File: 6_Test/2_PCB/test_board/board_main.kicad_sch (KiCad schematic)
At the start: 20 parts, among them J1 Power_Connector, J2 BNC_Odd, J3 BNC_Even, J4 Analog_Discovery_Inputs, J5 BNC_Inputs, J7 Digital_Supply_Jumpers, J8 Digital_Outputs, J9 Digital_Inputs

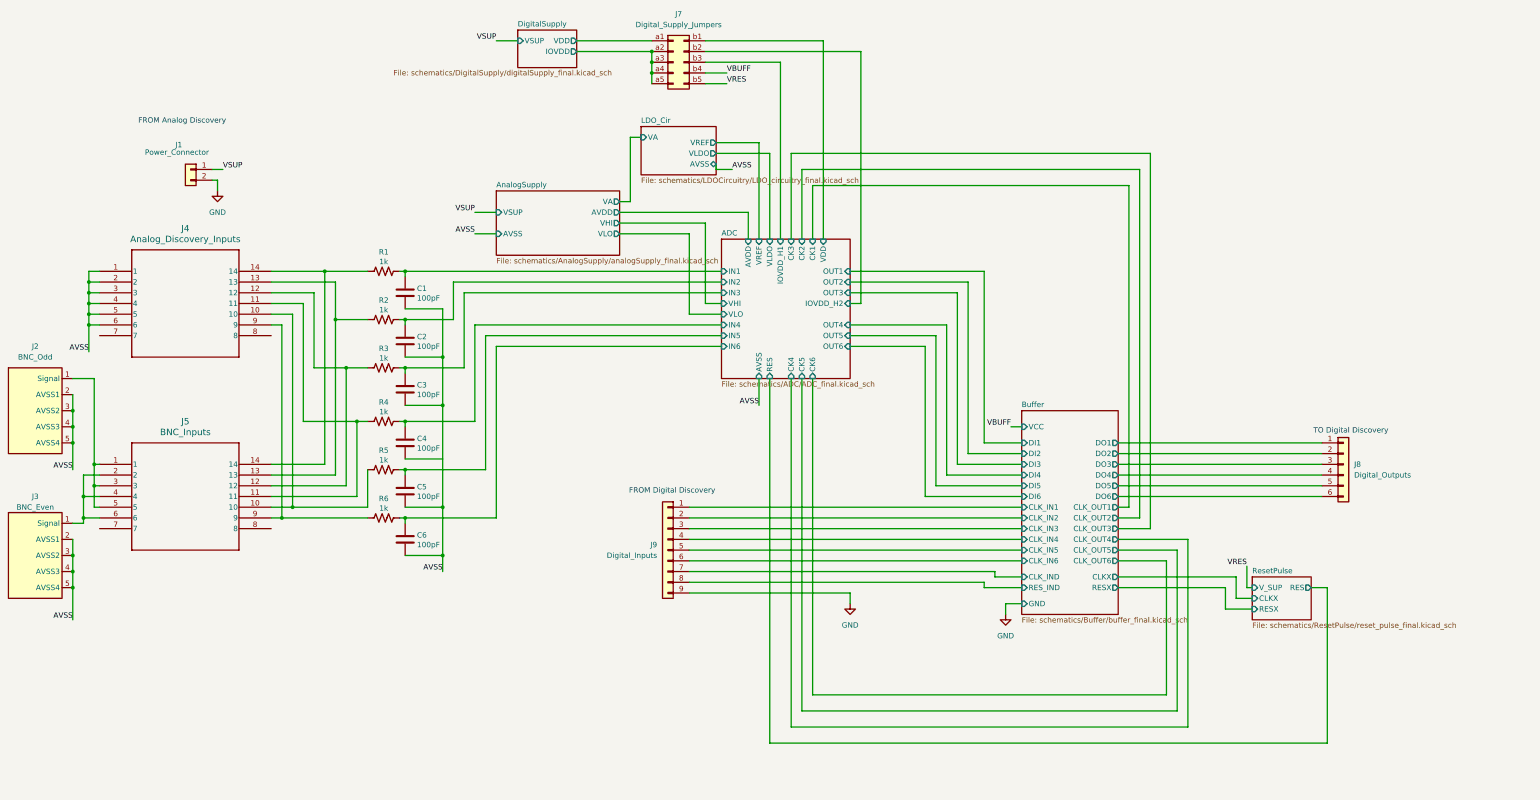
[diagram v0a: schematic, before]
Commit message: Adjusted Edits 11_25_24
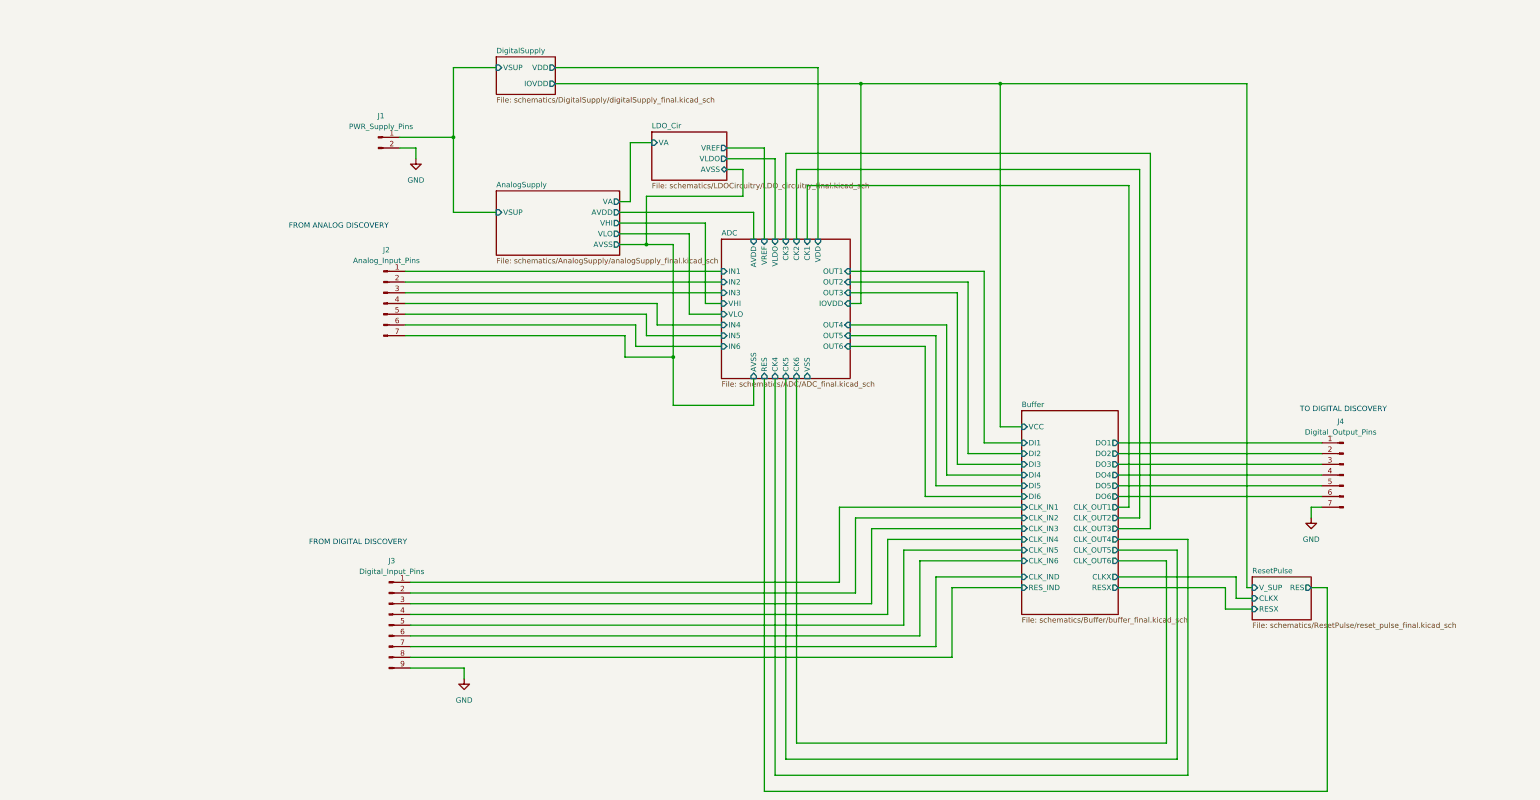
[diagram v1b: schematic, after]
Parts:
- removed C1, C2, C3, C4, C5, C6: 100pF, Capacitor_SMD:C_0201_0603Metric, symbol Device:C
- removed J1: Power_Connector, Connector_PinHeader_2.54mm:PinHeader_1x02_P2.54mm_Vertical, symbol Connector_Generic:Conn_01x02
- removed J2: BNC_Odd, symbol bnc_mini_with_gnd:bnc_mini_gnd
- removed J3: BNC_Even, symbol bnc_mini_with_gnd:bnc_mini_gnd
- removed J4: Analog_Discovery_Inputs, TSW-107-07-G-D_SAI, symbol 6x2Header:TSW-107-07-F-D
- removed J5: BNC_Inputs, TSW-107-07-G-D_SAI, symbol 6x2Header:TSW-107-07-F-D
- removed J7: Digital_Supply_Jumpers, Connector_PinHeader_2.54mm:PinHeader_2x05_P2.54mm_Vertical, symbol Connector_Generic:Conn_02x05_Row_Letter_First
- removed J8: Digital_Outputs, Connector_PinHeader_2.54mm:PinHeader_1x06_P2.54mm_Vertical, symbol Connector_Generic:Conn_01x06
- removed J9: Digital_Inputs, Connector_PinHeader_2.54mm:PinHeader_1x09_P2.54mm_Vertical, symbol Connector_Generic:Conn_01x09
- removed R1, R2, R3, R4, R5, R6: 1k, Resistor_SMD:R_0201_0603Metric, symbol Device:R_US
- added J1: PWR_Supply_Pins, Connector_PinHeader_2.54mm:PinHeader_1x02_P2.54mm_Vertical, symbol Connector:Conn_01x02_Pin
- added J2: Analog_Input_Pins, Connector_PinHeader_2.54mm:PinHeader_1x07_P2.54mm_Vertical, symbol Connector:Conn_01x07_Pin
- added J3: Digital_Input_Pins, Connector_PinHeader_2.54mm:PinHeader_1x09_P2.54mm_Vertical, symbol Connector:Conn_01x09_Pin
- added J4: Digital_Output_Pins, Connector_PinHeader_2.54mm:PinHeader_1x07_P2.54mm_Vertical, symbol Connector:Conn_01x07_Pin
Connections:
- net ADC/IN1: now also J2.1 (Pin_1)
- net ADC/IN2: now also J2.2 (Pin_2)
- net ADC/IN3: now also J2.3 (Pin_3)
- net ADC/IN4: now also J2.4 (Pin_4)
- net ADC/IN5: now also J2.5 (Pin_5)
- net ADC/IN6: now also J2.6 (Pin_6)
- net Buffer/CLK_IN1: now also J3.1 (Pin_1)
- net Buffer/CLK_IN2: now also J3.2 (Pin_2)
- net Buffer/CLK_IN3: now also J3.3 (Pin_3)
- net Buffer/CLK_IN4: now also J3.4 (Pin_4)
- net Buffer/CLK_IN5: now also J3.5 (Pin_5)
- net Buffer/CLK_IN6: now also J3.6 (Pin_6)
- net Buffer/CLK_IND: now also J3.7 (Pin_7)
- net Buffer/DO1: now also J4.1 (Pin_1)
- net Buffer/DO2: now also J4.2 (Pin_2)
- net Buffer/DO3: now also J4.3 (Pin_3)
- net Buffer/DO4: now also J4.4 (Pin_4)
- net Buffer/DO5: now also J4.5 (Pin_5)
- net Buffer/DO6: now also J4.6 (Pin_6)
- net Buffer/RES_IND: now also J3.8 (Pin_8)
- net GND: now also J1.2 (Pin_2), J3.9 (Pin_9), J4.7 (Pin_7)
- new net ADC/AVSS: J2.7 (Pin_7)
- new net AnalogSupply/VSUP: J1.1 (Pin_1)
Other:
- sheet ADC ports: added IOVDD, VSS; removed IOVDD_H1, IOVDD_H2
- sheet Buffer ports: added none; removed GND
- note added: "FROM ANALOG DISCOVERY"
- note added: "FROM DIGITAL DISCOVERY"
- note added: "TO DIGITAL DISCOVERY"
- note removed: "FROM Analog Discovery"
- note removed: "FROM Digital Discovery"
- note removed: "TO Digital Discovery"
